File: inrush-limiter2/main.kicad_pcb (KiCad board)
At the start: 2 copper layers, 31 parts, among them K1 RELAY_2RT, P1 CONN_01X04, Q1 2N3904, Q2 PN2222A, T1 TRANSFO, U1 LM393, U2 50 ohm NTC

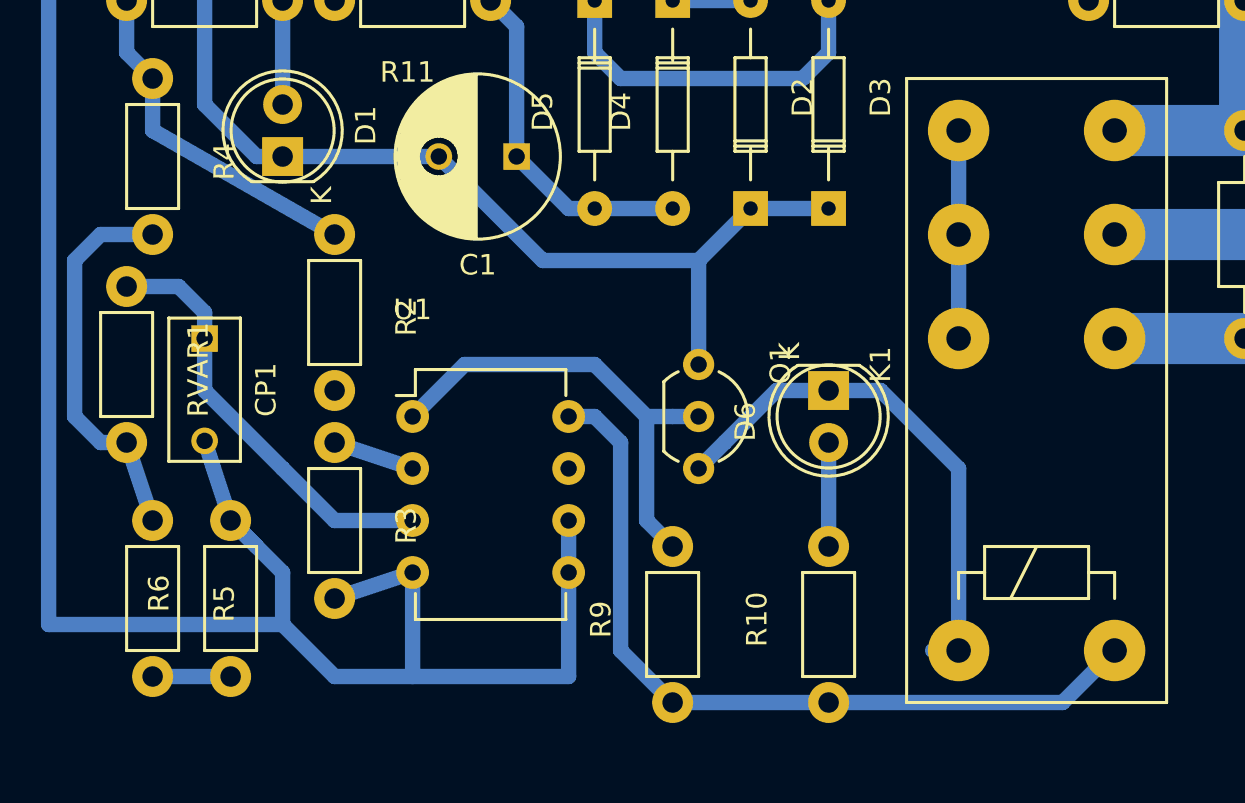
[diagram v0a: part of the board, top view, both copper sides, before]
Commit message: update
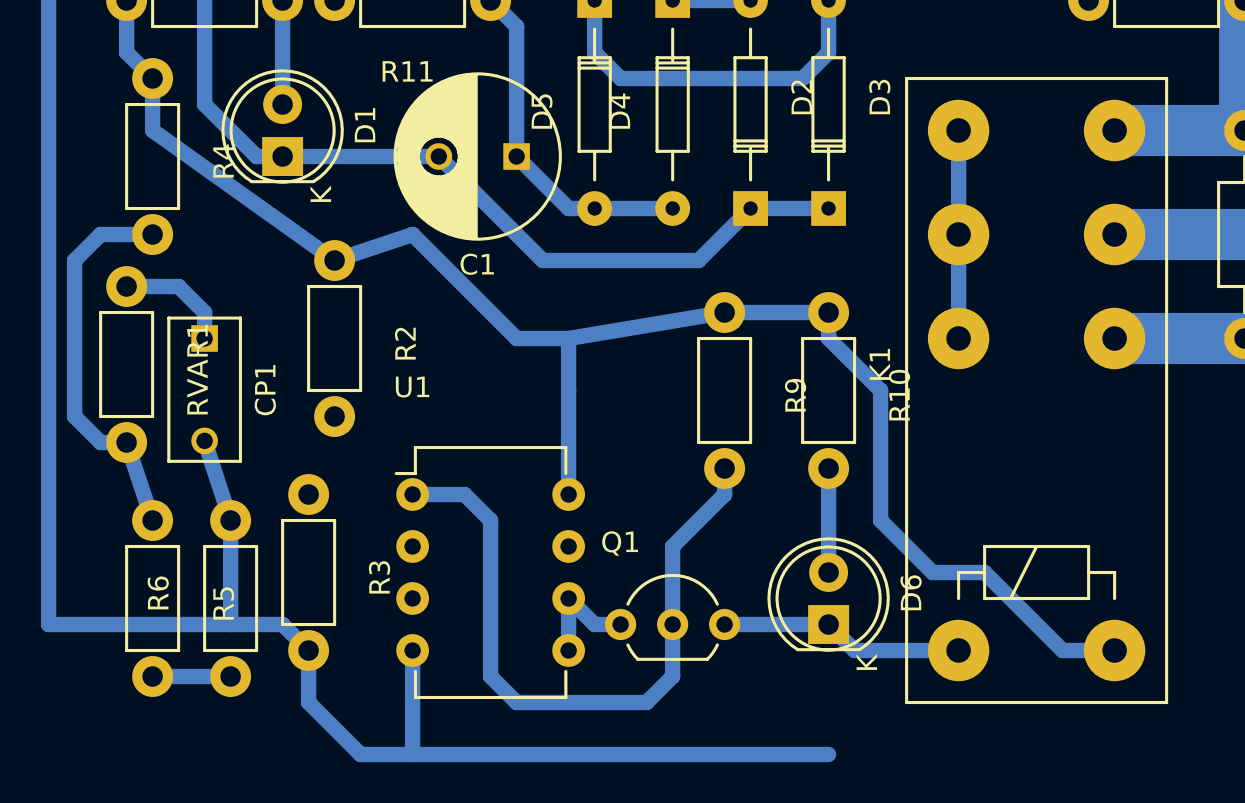
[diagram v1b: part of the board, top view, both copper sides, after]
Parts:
- moved R9 19.2 mm to (144.8, 74.9), turned to 270 degrees
- moved R10 19.0 mm to (149.9, 74.9), turned to 270 degrees
- moved Q1 13.3 mm to (139.7, 90.2), turned to 0 degrees
- moved D6 11.4 mm to (149.9, 90.2), turned to 90 degrees
- moved U1 3.81 mm to (129.5, 83.8)
- moved R3 2.84 mm to (124.5, 83.8)
- moved R2 1.27 mm to (125.7, 72.4)
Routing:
- net +5V: track 60.4 -> 81.0 mm
- net Net-(CP1-Pad1): track 20.9 -> 5.61 mm
- net Net-(D6-Pad1): track 26.0 -> 13.2 mm
- net Net-(Q1-Pad2): track 23.0 -> 33.1 mm
- net Net-(R2-Pad2): track 4.02 -> 0.00 mm
- net GND: track 175.8 -> 177.6 mm

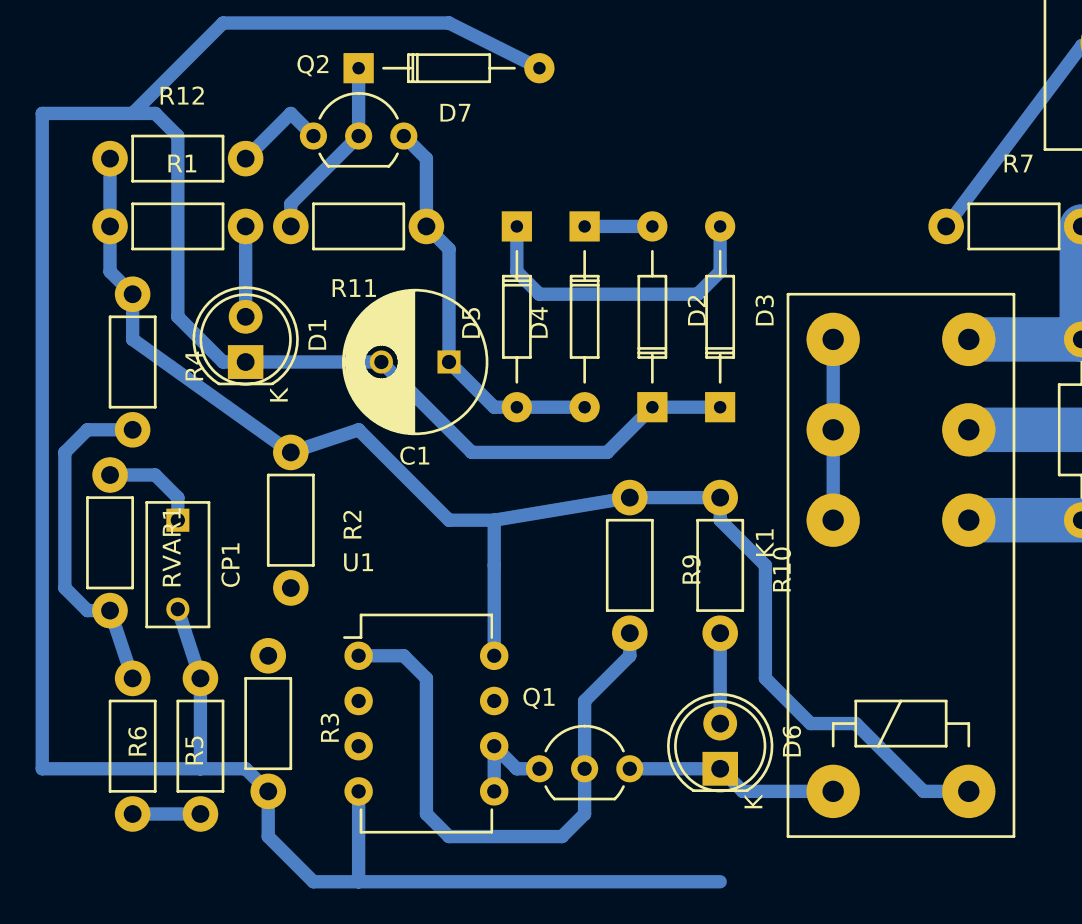
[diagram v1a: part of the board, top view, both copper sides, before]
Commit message: update
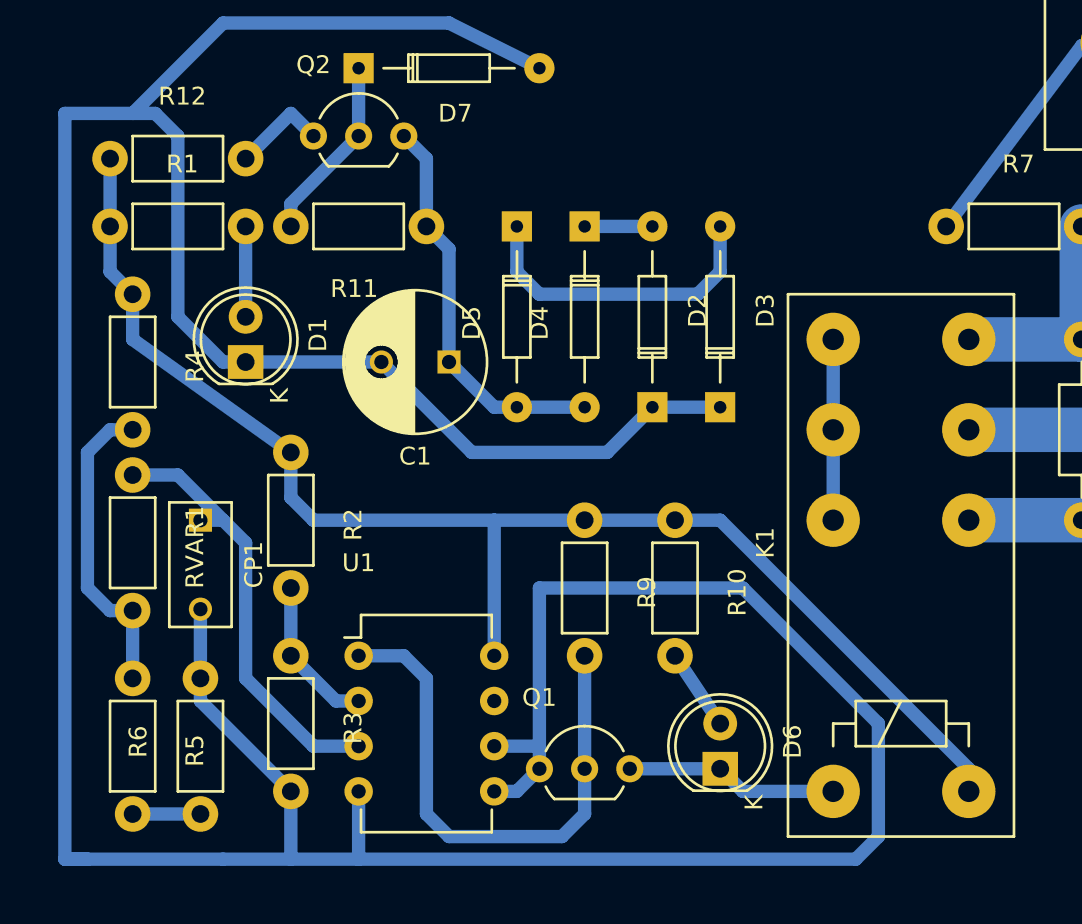
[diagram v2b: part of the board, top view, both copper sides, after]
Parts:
- moved R10 2.84 mm to (147.3, 76.2)
- moved R9 2.84 mm to (142.2, 76.2)
- moved CP1 1.27 mm to (120.7, 76.2)
- moved R3 1.27 mm to (125.7, 83.8)
- moved RVAR1 1.27 mm to (116.8, 73.7)
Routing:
- net GND: track 177.6 -> 231.2 mm
- net Net-(CP1-Pad1): track 5.61 -> 24.7 mm
- net Net-(R2-Pad2): track 0.00 -> 8.67 mm
- net +5V: track 81.0 -> 77.5 mm
- net Net-(Q1-Pad2): track 33.1 -> 30.8 mm
- net Net-(R4-Pad2): track 19.0 -> 17.6 mm
- net Net-(D6-Pad2): track 5.08 -> 4.58 mm
